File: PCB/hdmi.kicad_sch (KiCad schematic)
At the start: 25 parts, among them J3 HDMI-019S, U12 PCA9306DC1, U14 UCL0524P, U15 UCL0524P, U16 UCL0524P

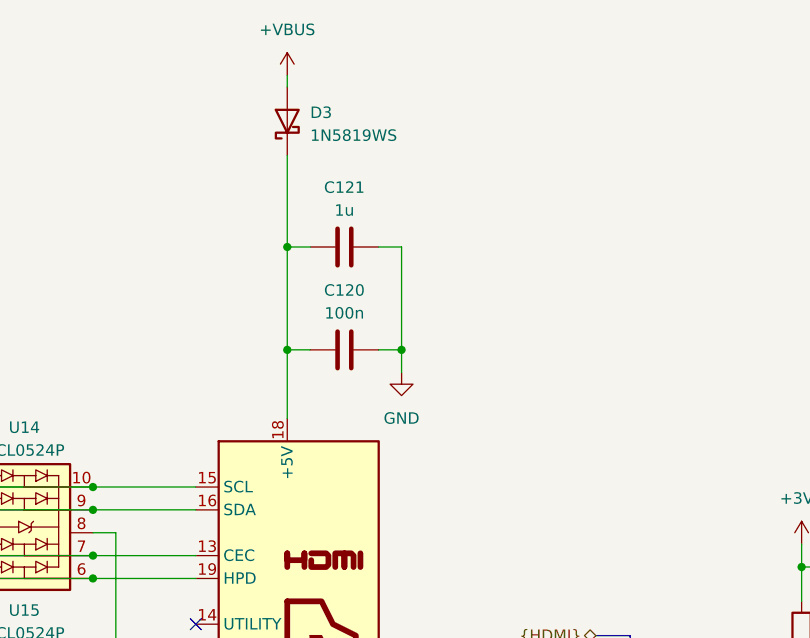
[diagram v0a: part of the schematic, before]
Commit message: cleaning  up the schematic some more before sharing
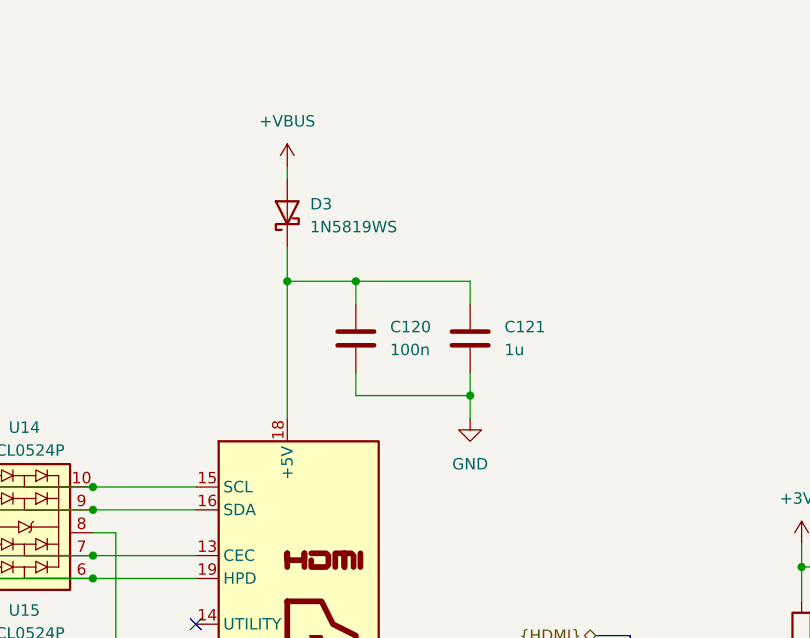
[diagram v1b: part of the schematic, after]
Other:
- moved on the sheet: D3

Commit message: added basic capacitor footprints
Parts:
- C113, C114, C115, C116, C117, C119, C120, C122, C123, C14, C16: footprint (none) -> Capacitor_SMD:C_0402_1005Metric
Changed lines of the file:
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@@
 			)
 		)
-		(property "Footprint" ""
+		(property "Footprint" "Capacitor_SMD:C_0402_1005Metric"
 			(at 73.66 110.49 0)
 			(effects
@@
 			)
 		)
-		(property "Footprint" ""
+		(property "Footprint" "Capacitor_SMD:C_0402_1005Metric"
 			(at 67.31 115.57 0)
 			(effects
@@
 			)
 		)
-		(property "Footprint" ""
+		(property "Footprint" "Capacitor_SMD:C_0402_1005Metric"
 			(at 67.31 123.19 0)
 			(effects
@@
 			)
 		)
-		(property "Footprint" ""
+		(property "Footprint" "Capacitor_SMD:C_0402_1005Metric"
 			(at 202.8952 105.41 0)
 			(effects
@@
 			)
 		)
-		(property "Footprint" ""
+		(property "Footprint" "Capacitor_SMD:C_0402_1005Metric"
 			(at 67.31 107.95 0)
 			(effects
@@
 			)
 		)
-		(property "Footprint" ""
+		(property "Footprint" "Capacitor_SMD:C_0402_1005Metric"
 			(at 73.66 118.11 0)
 			(effects
@@
 			)
 		)
-		(property "Footprint" ""
+		(property "Footprint" "Capacitor_SMD:C_0402_1005Metric"
 			(at 134.3152 74.93 0)
 			(effects
@@
 			)
 		)
-		(property "Footprint" ""
+		(property "Footprint" "Capacitor_SMD:C_0402_1005Metric"
 			(at 237.1852 105.41 0)
 			(effects
@@
 			)
 		)
-		(property "Footprint" ""
+		(property "Footprint" "Capacitor_SMD:C_0402_1005Metric"
 			(at 73.66 125.73 0)
 			(effects
@@
 			)
 		)
-		(property "Footprint" ""
+		(property "Footprint" "Capacitor_SMD:C_0402_1005Metric"
 			(at 73.66 133.35 0)
 			(effects
@@
 			)
 		)
-		(property "Footprint" ""
+		(property "Footprint" "Capacitor_SMD:C_0402_1005Metric"
 			(at 67.31 130.81 0)
 			(effects

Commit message: finisehed upassigning resistor footprints
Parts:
- R47: footprint (none) -> Resistor_SMD:R_0603_1608Metric
- R57, R58, R59, R60, R61, R62: footprint (none) -> Resistor_SMD:R_0402_1005Metric
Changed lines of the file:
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@@
 			)
 		)
-		(property "Footprint" ""
+		(property "Footprint" "Resistor_SMD:R_0402_1005Metric"
 			(at 189.992 104.14 90)
 			(effects
@@
 			)
 		)
-		(property "Footprint" ""
+		(property "Footprint" "Resistor_SMD:R_0402_1005Metric"
 			(at 67.31 99.568 90)
 			(effects
@@
 			)
 		)
-		(property "Footprint" ""
+		(property "Footprint" "Resistor_SMD:R_0402_1005Metric"
 			(at 249.682 104.14 90)
 			(effects
@@
 			)
 		)
-		(property "Footprint" ""
+		(property "Footprint" "Resistor_SMD:R_0402_1005Metric"
 			(at 258.572 104.14 90)
 			(effects
@@
 			)
 		)
-		(property "Footprint" ""
+		(property "Footprint" "Resistor_SMD:R_0402_1005Metric"
 			(at 181.102 104.14 90)
 			(effects
@@
 			)
 		)
-		(property "Footprint" ""
+		(property "Footprint" "Resistor_SMD:R_0402_1005Metric"
 			(at 243.84 94.742 90)
 			(effects
@@
 			)
 		)
-		(property "Footprint" ""
+		(property "Footprint" "Resistor_SMD:R_0603_1608Metric"
 			(at 56.642 78.74 90)
 			(effects
